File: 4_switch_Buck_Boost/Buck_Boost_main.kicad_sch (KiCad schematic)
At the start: 58 parts, among them J1 Screw_Terminal_2x5.08, J2 Screw_Terminal_2x5.08, J3 Screw_Terminal_2x2.54, Q1 CSD18532Q5B, Q101 2N7002K, Q103 BSS83P, Q2 CSD18532Q5B, Q3 CSD18532Q5B, Q4 CSD18532Q5B, U1 LT8390EUFD_PBF

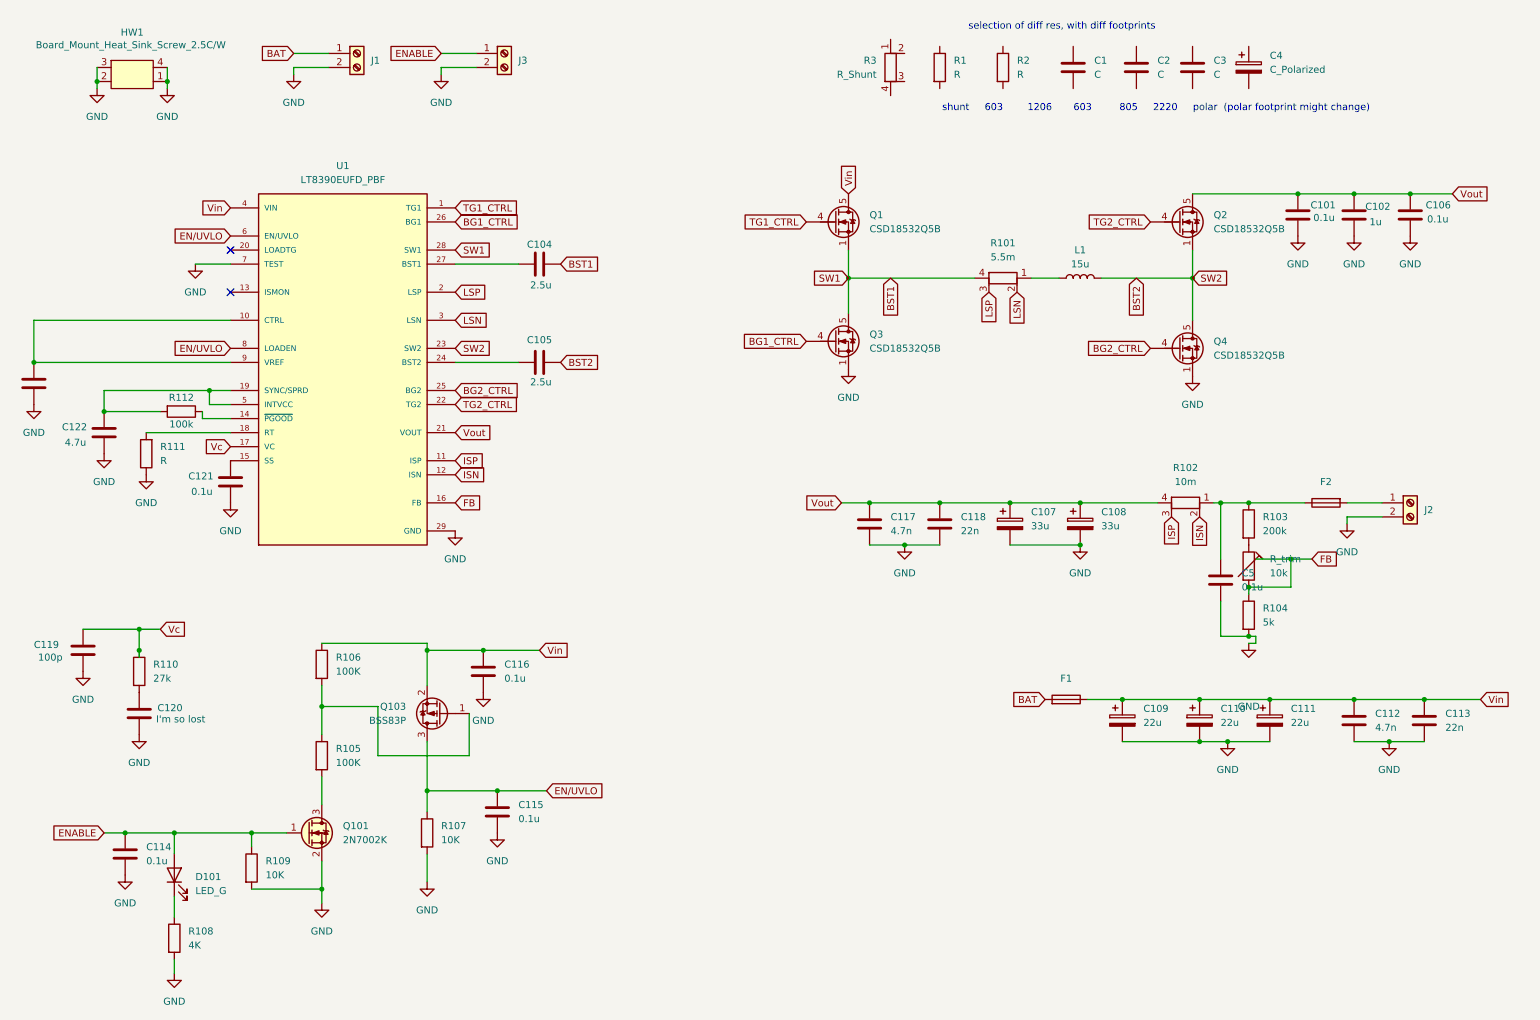
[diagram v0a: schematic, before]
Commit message: finish up schematic before final check
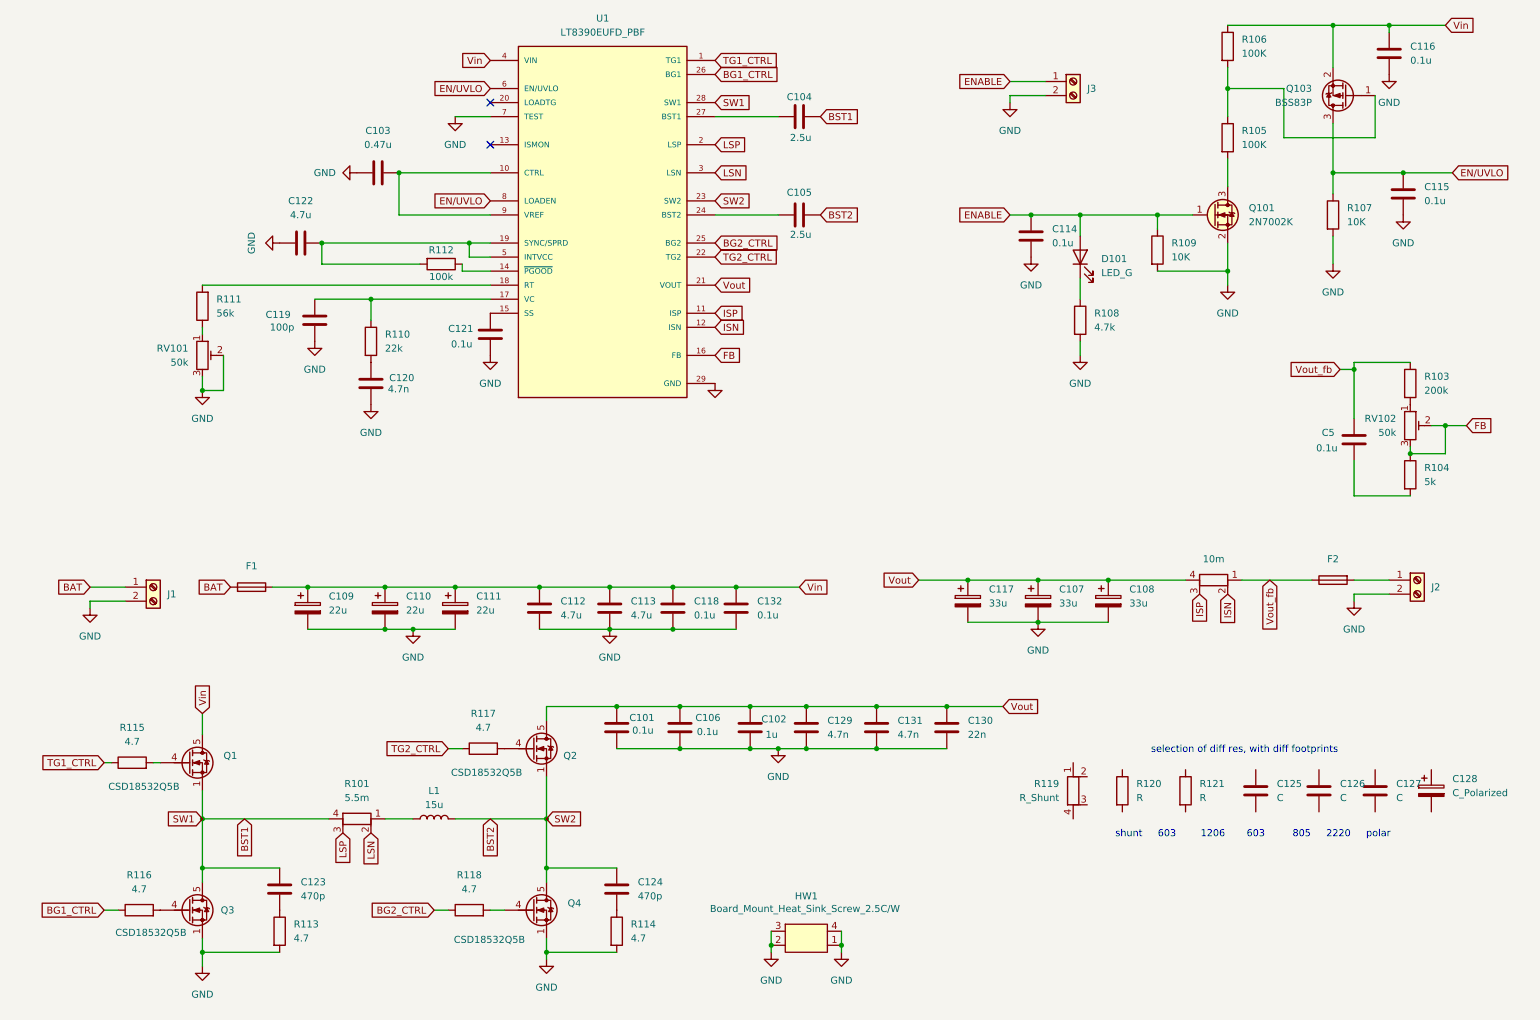
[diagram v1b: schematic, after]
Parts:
- removed C1: C, rsx_capacitors:C_0603_1608Metric, symbol Device:C
- removed C117: 4.7n, rsx_capacitors:C_0603_1608Metric, symbol Device:C
- removed C2: C, rsx_capacitors:C_0805_2012Metric, symbol Device:C
- removed C3: C, rsx_capacitors:C_2220_5750Metric_Pad1.97x5.40mm_HandSolder, symbol Device:C
- removed C4: C_Polarized, Capacitor_SMD:CP_Elec_8x10.5, symbol Device:C_Polarized
- removed R1: R, rsx_resistors:R_0603_1608Metric, symbol Device:R
- removed R2: R, rsx_resistors:R_1206_3216Metric, symbol Device:R
- removed R3: R_Shunt, Resistor_SMD:R_Shunt_Vishay_WSK2512_6332Metric_T1.19mm, symbol Device:R_Shunt
- removed R_trim: 10k, symbol Device:R_Trim
- added C117: 33u, Capacitor_SMD:CP_Elec_8x10.5, symbol Device:C_Polarized
- added C123, C124: 470p, rsx_capacitors:C_0603_1608Metric, symbol Device:C
- added C125: C, rsx_capacitors:C_0603_1608Metric, symbol Device:C
- added C126: C, rsx_capacitors:C_0805_2012Metric, symbol Device:C
- added C127: C, rsx_capacitors:C_2220_5750Metric_Pad1.97x5.40mm_HandSolder, symbol Device:C
- added C128: C_Polarized, Capacitor_SMD:CP_Elec_8x10.5, symbol Device:C_Polarized
- added C129, C131: 4.7n, rsx_capacitors:C_0603_1608Metric, symbol Device:C
- added C130: 22n, rsx_capacitors:C_0603_1608Metric, symbol Device:C
- added C132: 0.1u, rsx_capacitors:C_0603_1608Metric, symbol Device:C
- added R113, R114, R115, R116, R117, R118: 4.7, rsx_resistors:R_0603_1608Metric, symbol Device:R
- added R119: R_Shunt, Resistor_SMD:R_Shunt_Vishay_WSK2512_6332Metric_T1.19mm, symbol Device:R_Shunt
- added R120: R, rsx_resistors:R_0603_1608Metric, symbol Device:R
- added R121: R, rsx_resistors:R_1206_3216Metric, symbol Device:R
- added RV101, RV102: 50k, rsx_resistors:Potentiometer_Bourns_3296W_Vertical_DL, symbol Device:R_Potentiometer_Trim
- C103: value 4.7uF -> 0.47u
- C112: value 4.7n -> 4.7u; footprint rsx_capacitors:C_0603_1608Metric -> rsx_capacitors:C_0805_2012Metric
- C113: value 22n -> 4.7u; footprint rsx_capacitors:C_0603_1608Metric -> rsx_capacitors:C_0805_2012Metric
- C118: value 22n -> 0.1u
- C120: value I'm so lost -> 4.7n
- C122: footprint rsx_capacitors:C_0603_1608Metric -> rsx_capacitors:C_0805_2012Metric
- R108: value 4K -> 4.7k
- R110: value 27k -> 22k
- R111: value R -> 56k
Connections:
- net BG1_CTRL: now also R116.1; no longer Q3.4 (G)
- net BG2_CTRL: now also R118.1; no longer Q4.4 (G)
- net BST1: now also C123.1
- net BST2: now also C124.1
- net FB: now also RV102.2, RV102.3
- net GND: now also C103.1, C122.1, C117.2, C129.2, C130.2, C131.2, C132.2, R113.2, R114.2, RV101.2, RV101.3; no longer C103.2, C122.2, C5.2, R104.2, R111.1
- net TG1_CTRL: now also R115.1; no longer Q1.4 (G)
- net TG2_CTRL: now also R117.1; no longer Q2.4 (G)
- net Vin: now also C118.1, C132.1
- net Vout: now also C117.1, C129.1, C130.1, C131.1; no longer C118.1
- net Vout_fb: now reaches C5.1, F2.2, R102.1, R103.1
- net at R112.2, U1.19 (SYNC/SPRD), U1.5 (INTVCC): now also C122.2; no longer C122.1
- net at U1.10 (CTRL), U1.9 (VREF): now also C103.2; no longer C103.1
- net at R103.2: now also RV102.1
- net Vc: no longer names the net of C119.1, R110.1, U1.17 (VC)
- new net: Q3.4 (G), R116.2
- new net: C124.2, R114.1
- new net: C123.2, R113.1
- new net: Q4.4 (G), R118.2
- new net: C5.2, R104.2
- new net: Q1.4 (G), R115.2
- new net: R111.1, RV101.1
- new net: Q2.4 (G), R117.2
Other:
- note added: "shunt 603 1206 603 805 2220 polar"
- note removed: "shunt 603 1206 603 805 2220 polar (polar footprint might change)"
- moved on the sheet: C101, C102, C104, C105, C106, C107, C108, C109, C110, C111, C114, C115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
